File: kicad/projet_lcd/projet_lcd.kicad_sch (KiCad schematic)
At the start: 49 parts, among them U1 KMS-1102NL, U2 LAN8742A-CZ-TR, Y1 25MHz

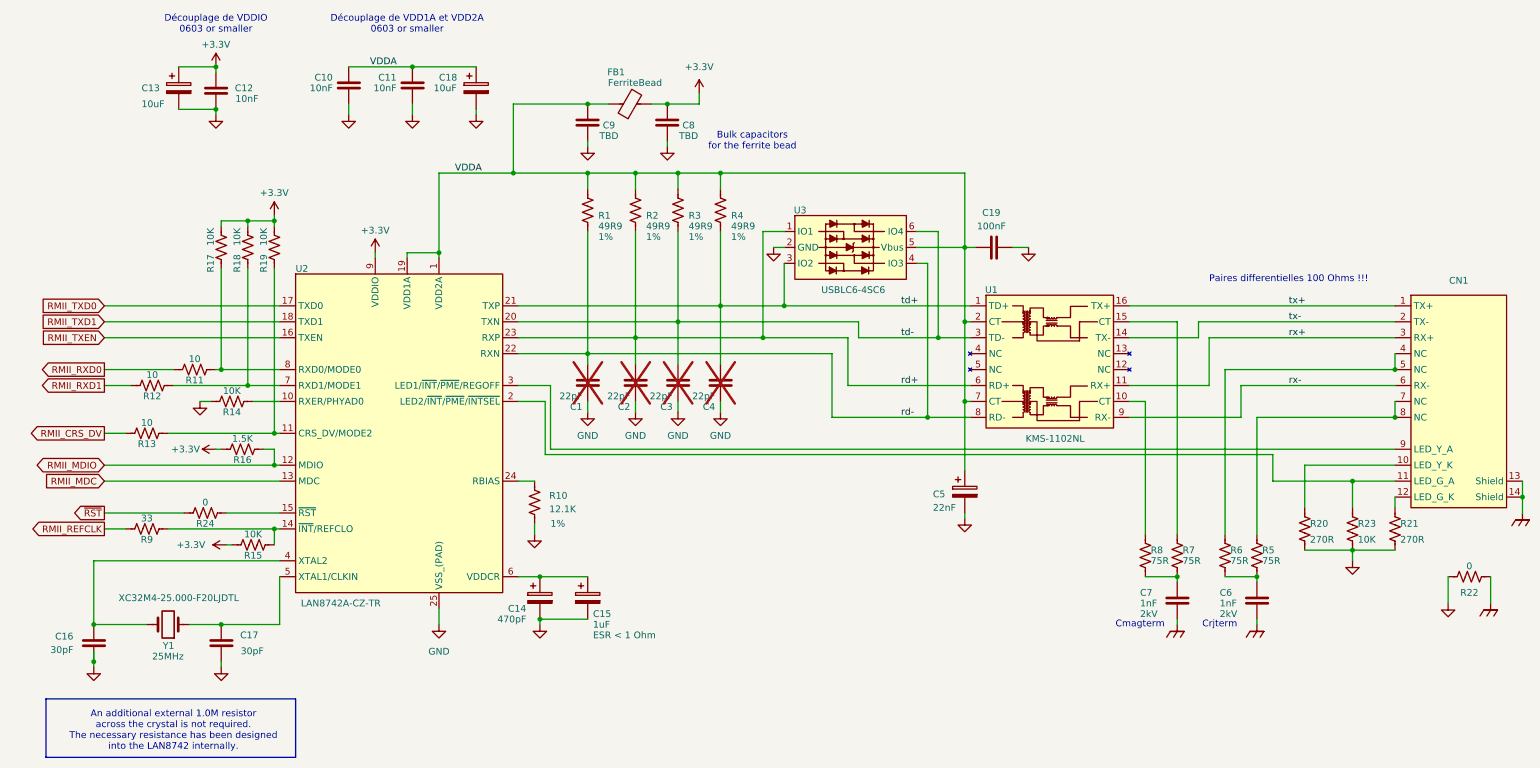
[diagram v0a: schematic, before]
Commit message: Work in progress
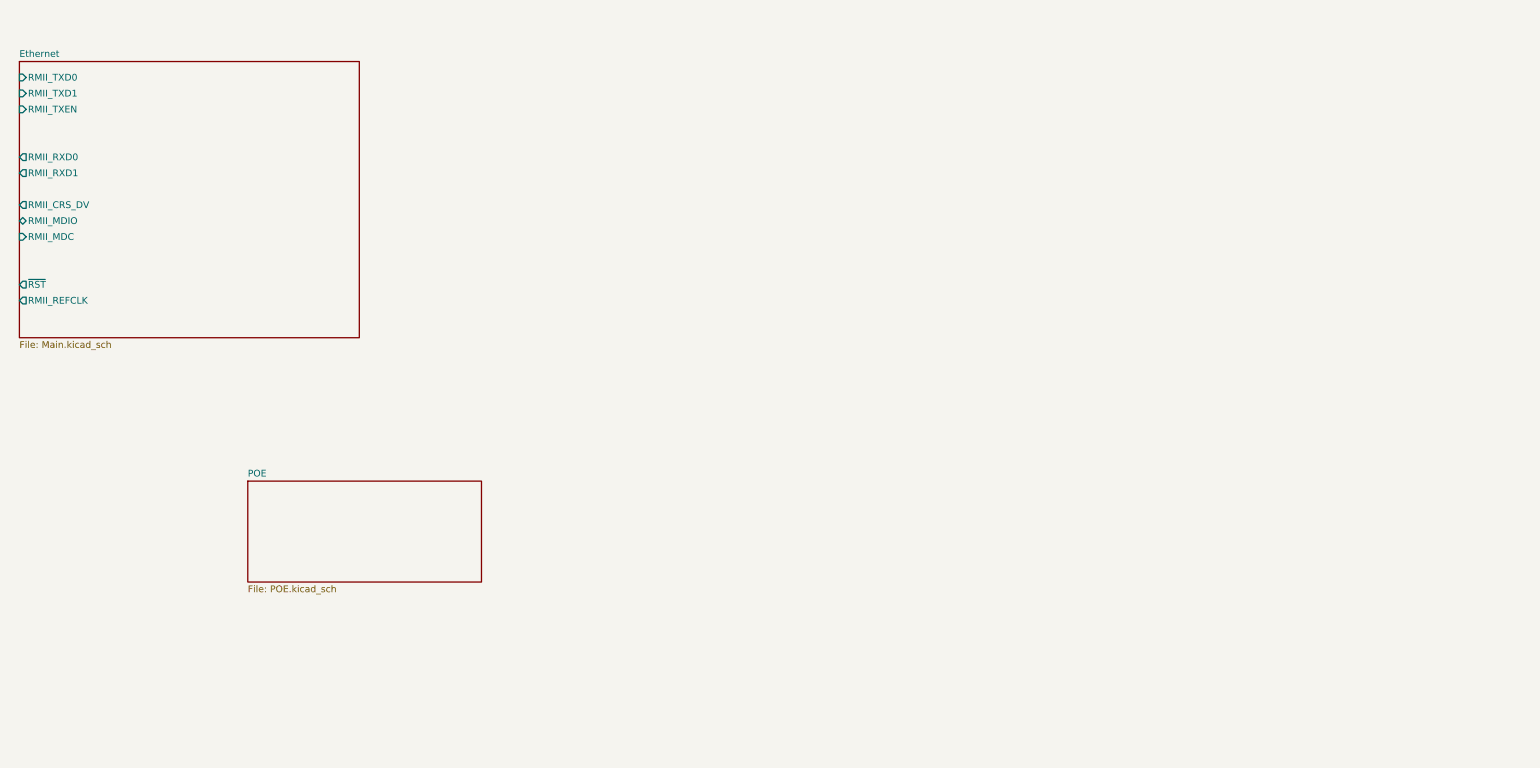
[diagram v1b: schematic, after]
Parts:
- removed C1, C2, C3, C4: 22pF, symbol Generiques:C
- removed C10, C11, C12: 10nF, symbol Generiques:C
- removed C13, C18: 10uF, symbol Generiques:C_Polarized
- removed C14: 470pF, symbol Generiques:C_Polarized
- removed C15: 1uF, symbol Generiques:C_Polarized
- removed C16, C17: 30pF, symbol Generiques:C
- removed C19: 100nF, symbol Generiques:C
- removed C5: 22nF, symbol Generiques:C_Polarized
- removed C6, C7: 1nF, symbol Generiques:C
- removed C8, C9: TBD, symbol Generiques:C
- removed CN1: ~, symbol Connectors:RJ45_with_Leds
- removed FB1: FerriteBead, symbol Generiques:FerriteBead
- removed R1, R2, R3, R4: 49R9, symbol Generiques:R
- removed R10: 12.1K, symbol Generiques:R
- removed R11, R12, R13: 10, symbol Generiques:R
- removed R14, R15, R17, R18, R19, R23: 10K, symbol Generiques:R
- removed R16: 1.5K, symbol Generiques:R
- removed R20, R21: 270R, symbol Generiques:R
- removed R22, R24: 0, symbol Generiques:R
- removed R5, R6, R7, R8: 75R, symbol Generiques:R
- removed R9: 33, symbol Generiques:R
- removed U1: KMS-1102NL, symbol Divers:KMS-1102NL
- removed U2: LAN8742A-CZ-TR, symbol Chips:LAN8742A
- removed U3: ~, symbol Diodes:USBLC6-4
- removed Y1: 25MHz, symbol Generiques:Crystal
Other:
- added sheet Ethernet (Main.kicad_sch)
- added sheet POE (POE.kicad_sch)
- note removed: "An additional external 1.0M resistor across the crystal is not required. The necessary resistance has been designed into the LAN8742 internally."
- note removed: "Bulk capacitors for the ferrite bead"
- note removed: "Cmagterm"
- note removed: "Crjterm"
- note removed: "Découplage de VDD1A et VDD2A 0603 or smaller"
- note removed: "Découplage de VDDIO 0603 or smaller"
- note removed: "Paires differentielles 100 Ohms !!!"
